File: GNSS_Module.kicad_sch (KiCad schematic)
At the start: 30 parts, among them J2 FTDI_Conn, J4 GPS_Conn, J9 GPS_Conn, U11 ublox_SAM-M8Q

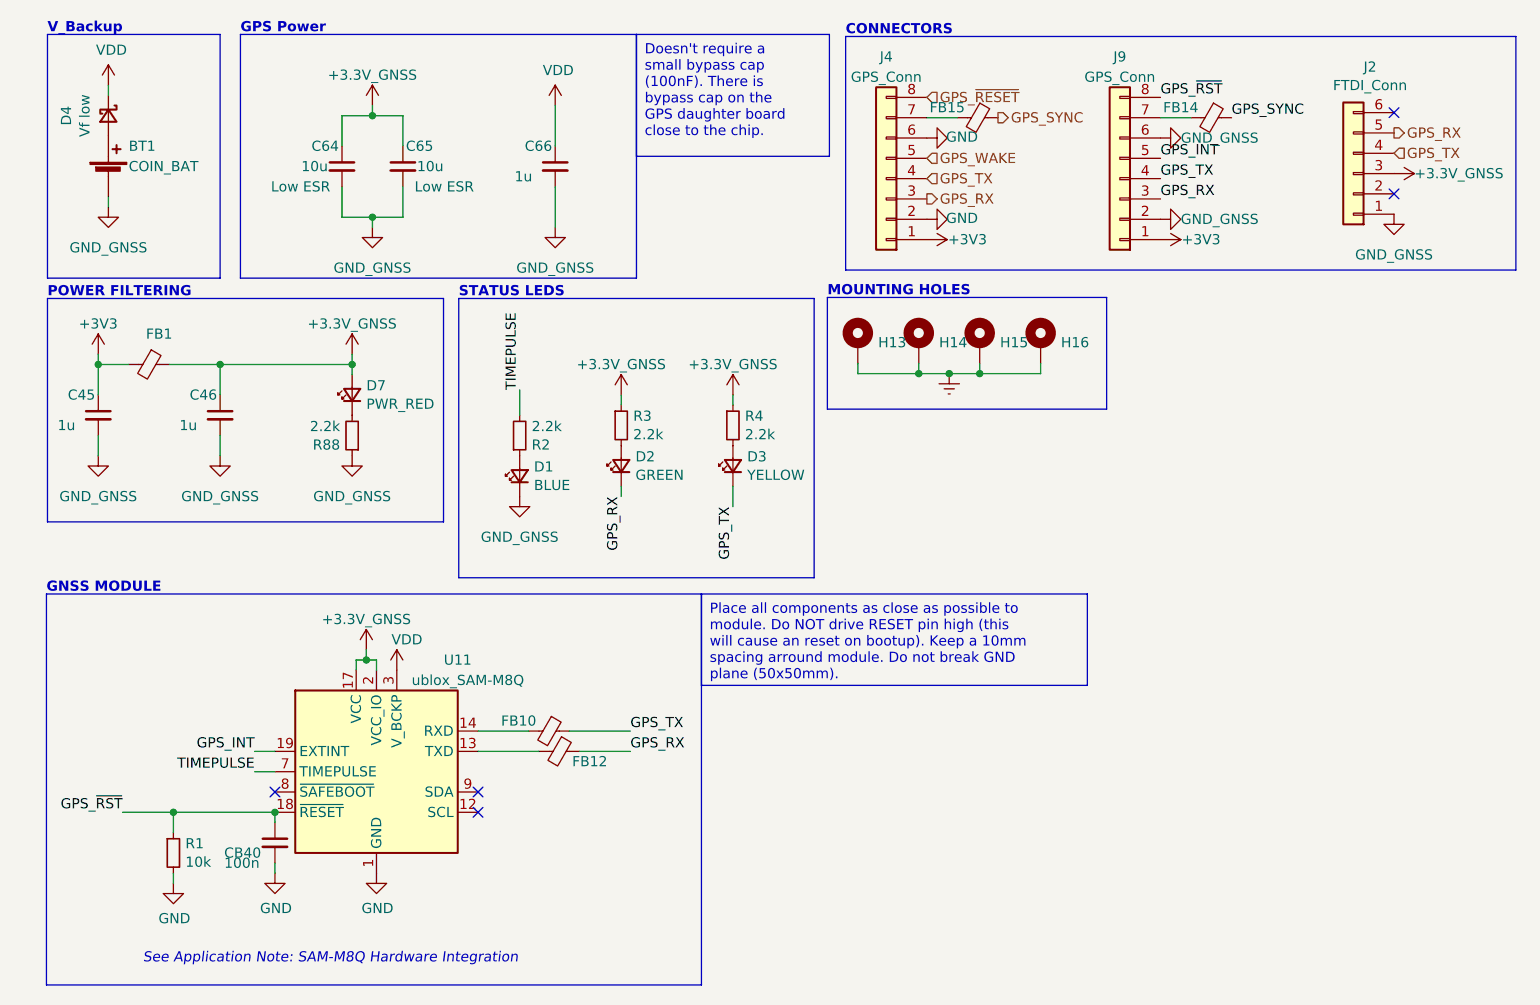
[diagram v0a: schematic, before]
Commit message: (bc) changes for the day
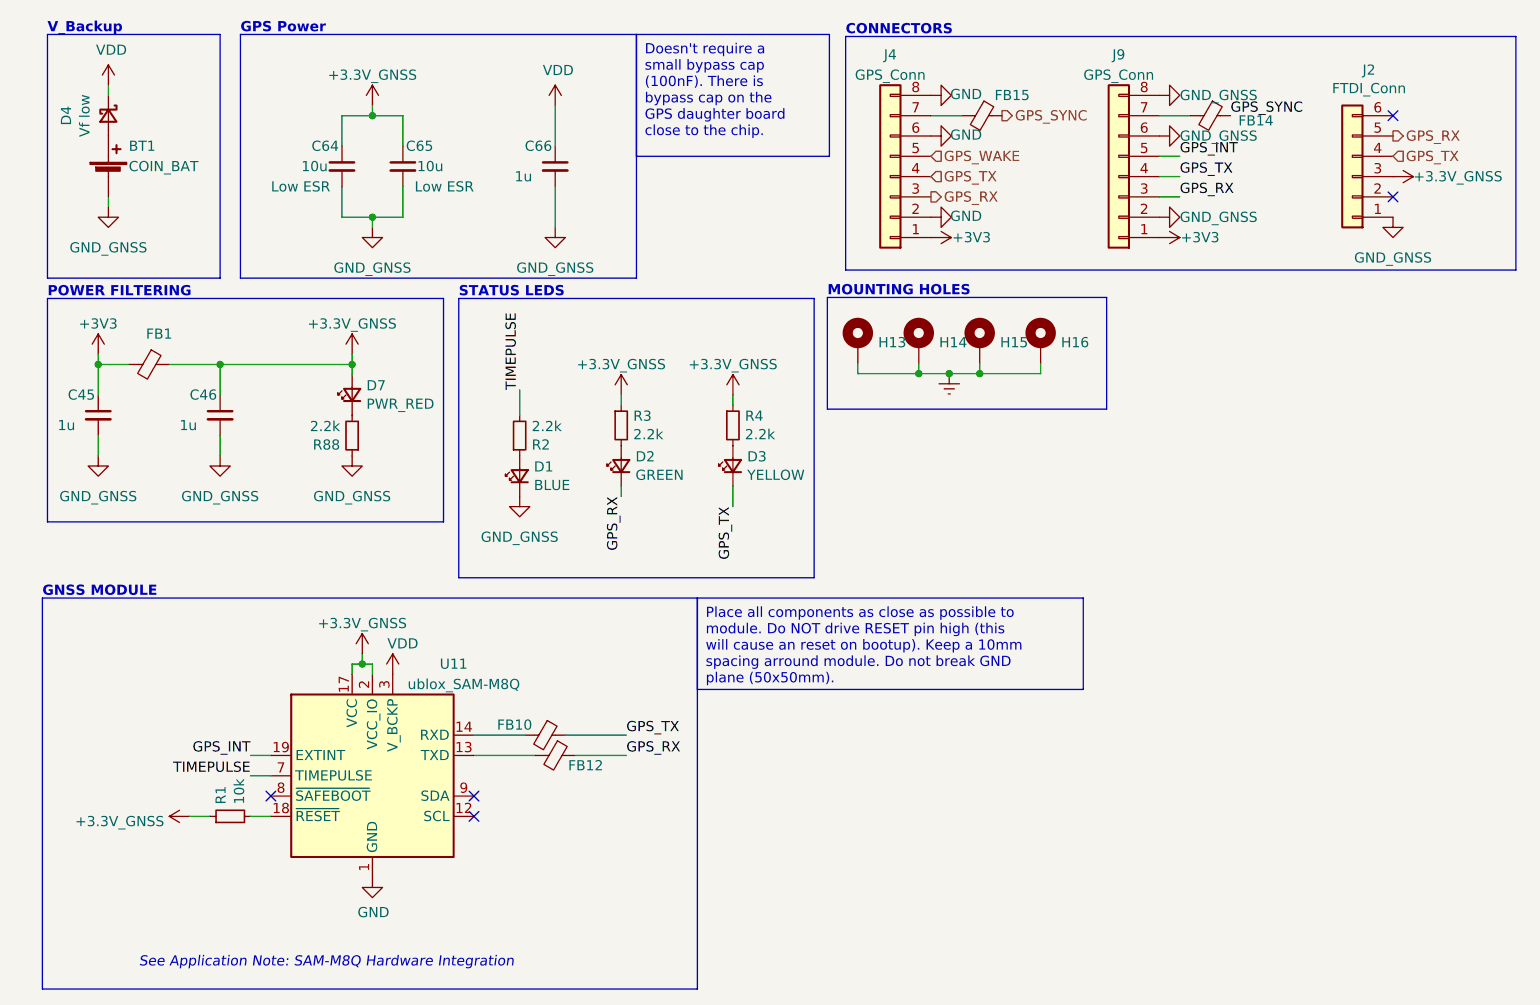
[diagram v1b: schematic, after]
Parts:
- removed CB40: 100n, Capacitor_SMD:C_0603_1608Metric_Pad1.08x0.95mm_HandSolder, symbol Device:C_Small
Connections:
- net GPS_~{RESET} is gone; now on net GND: J4.8 (Pin_8)
- net +3.3V: now also R1.1
- net GND: now also J9.8 (Pin_8); no longer R1.2
- removed net GPS_~{RST}: J9.8 (Pin_8), R1.1, U11.18 (~{RESET})
- new net: R1.2, U11.18 (~{RESET})
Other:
- moved on the sheet: FB10, FB12, FB15, J4, R1, U11
